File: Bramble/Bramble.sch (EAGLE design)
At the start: 15 parts, among them J3 5787745-1, J4 5787745-1

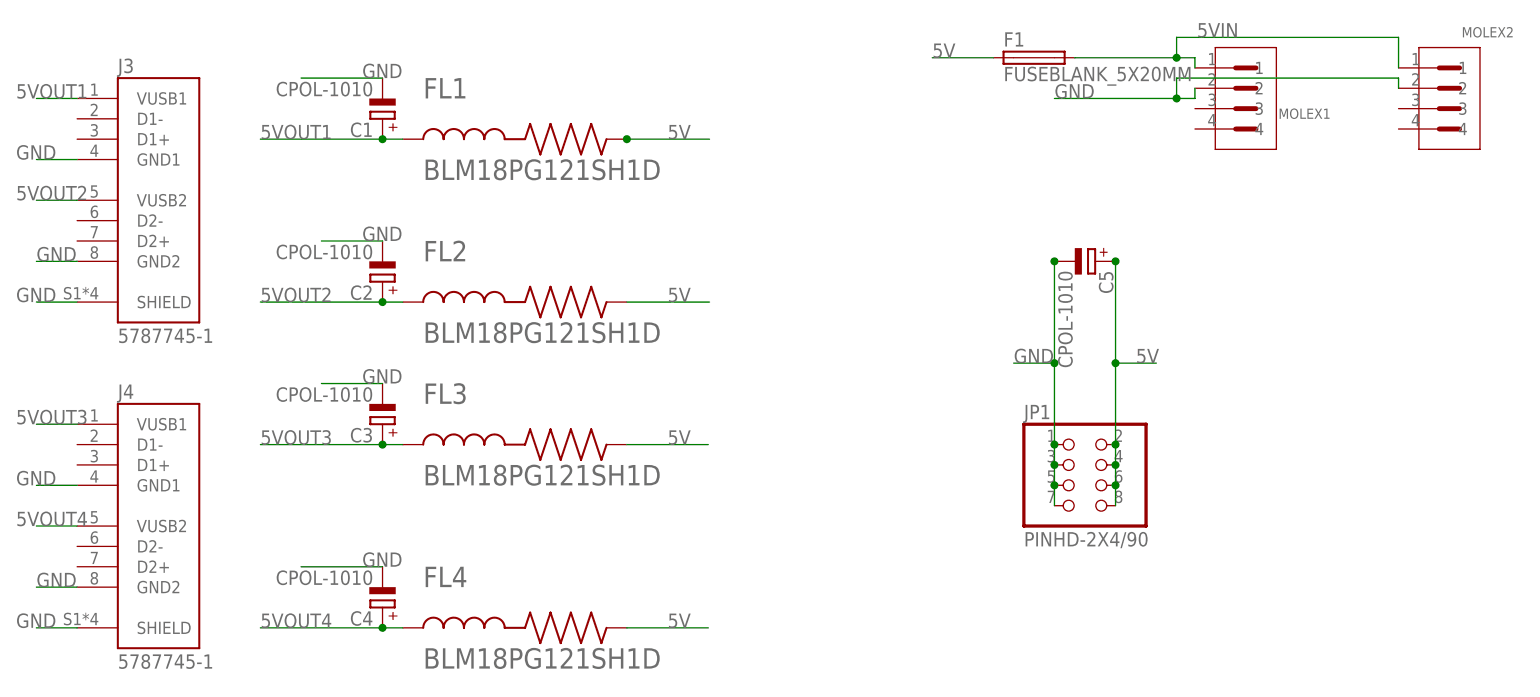
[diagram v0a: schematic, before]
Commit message: joined 1 and 2  aaand 3 and 4
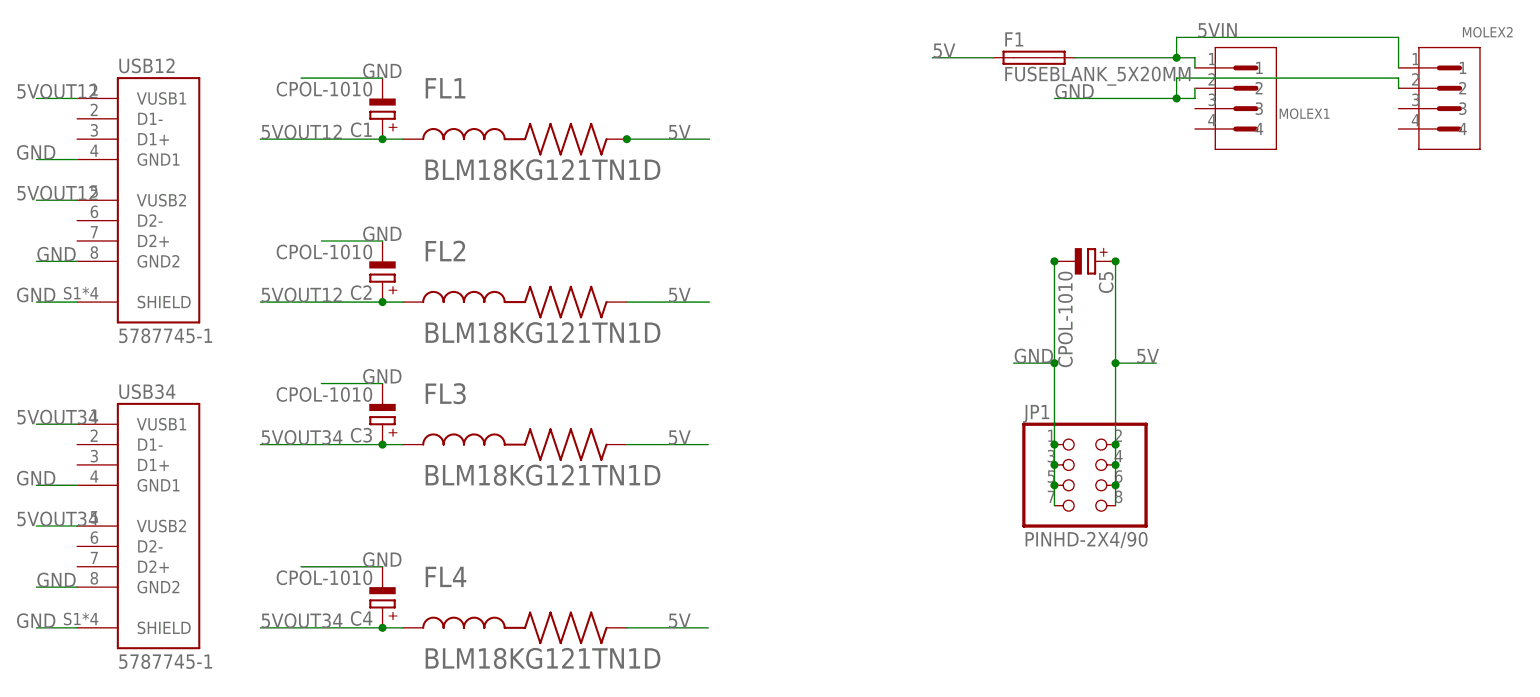
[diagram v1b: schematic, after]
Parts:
- FL1, FL2, FL3, FL4: value BLM18PG121SH1D -> BLM18KG121TN1D
- renumbered J3 to USB12, J4 to USB34
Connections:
- removed net 5VOUT1: C1.+, FL1.1, USB12.VUSB1
- removed net 5VOUT2: C2.+, FL2.1, USB12.VUSB2
- removed net 5VOUT3: C3.+, FL3.1, USB34.VUSB1
- removed net 5VOUT4: C4.+, FL4.1, USB34.VUSB2
- new net 5VOUT12: C1.+, C2.+, FL1.1, FL2.1, USB12.VUSB1, USB12.VUSB2
- new net 5VOUT34: C3.+, C4.+, FL3.1, FL4.1, USB34.VUSB1, USB34.VUSB2
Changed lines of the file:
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@@
 <part name="C4" library="cap-vishay-153clv" deviceset="CPOL-1010" device=""/>
 <part name="C5" library="cap-vishay-153clv" deviceset="CPOL-1010" device=""/>
-<part name="FL1" library="BLM18PG121SH1D" deviceset="BLM18PG121SH1D" device=""/>
-<part name="FL2" library="BLM18PG121SH1D" deviceset="BLM18PG121SH1D" device=""/>
-<part name="FL3" library="BLM18PG121SH1D" deviceset="BLM18PG121SH1D" device=""/>
-<part name="FL4" library="BLM18PG121SH1D" deviceset="BLM18PG121SH1D" device=""/>
+<part name="FL1" library="BLM18PG121SH1D" deviceset="BLM18PG121SH1D" device="" value="BLM18KG121TN1D"/>
+<part name="FL2" library="BLM18PG121SH1D" deviceset="BLM18PG121SH1D" device="" value="BLM18KG121TN1D"/>
+<part name="FL3" library="BLM18PG121SH1D" deviceset="BLM18PG121SH1D" device="" value="BLM18KG121TN1D"/>
+<part name="FL4" library="BLM18PG121SH1D" deviceset="BLM18PG121SH1D" device="" value="BLM18KG121TN1D"/>
 <part name="MOLEX1" library="15244441" deviceset="15244441" device=""/>
 <part name="MOLEX2" library="15244441" deviceset="15244441" device=""/>
-<part name="J3" library="5787745-1" deviceset="5787745-1" device=""/>
-<part name="J4" library="5787745-1" deviceset="5787745-1" device=""/>
+<part name="USB12" library="5787745-1" deviceset="5787745-1" device=""/>
+<part name="USB34" library="5787745-1" deviceset="5787745-1" device=""/>
 </parts>
 <sheets>
@@
 <attribute name="NAME" x="142.23916875" y="76.201240625" size="1.270209375" layer="95"/>
 </instance>
-<instance part="J3" gate="G$1" x="-20.32" y="55.88" smashed="yes">
+<instance part="USB12" gate="G$1" x="-20.32" y="55.88" smashed="yes">
 <attribute name="NAME" x="-25.400109375" y="71.7553" size="1.778040625" layer="95"/>
 <attribute name="VALUE" x="-25.40351875" y="38.0877" size="1.77923125" layer="96"/>
 </instance>
-<instance part="J4" gate="G$1" x="-20.32" y="15.24" smashed="yes">
+<instance part="USB34" gate="G$1" x="-20.32" y="15.24" smashed="yes">
 <attribute name="NAME" x="-25.400109375" y="31.1153" size="1.778040625" layer="95"/>
 <attribute name="VALUE" x="-25.40351875" y="-2.5523" size="1.77923125" layer="96"/>
@@
 <segment>
 <wire x1="-35.56" y1="43.18" x2="-30.48" y2="43.18" width="0.1524" layer="91"/>
-<pinref part="J3" gate="G$1" pin="SHIELD"/>
+<pinref part="USB12" gate="G$1" pin="SHIELD"/>
 <label x="-38.1" y="43.18" size="1.778" layer="95"/>
 </segment>
 <segment>
 <wire x1="-35.56" y1="2.54" x2="-30.48" y2="2.54" width="0.1524" layer="91"/>
-<pinref part="J4" gate="G$1" pin="SHIELD"/>
+<pinref part="USB34" gate="G$1" pin="SHIELD"/>
 <label x="-38.1" y="2.54" size="1.778" layer="95"/>
 </segment>
 <segment>
 <wire x1="-35.56" y1="20.32" x2="-30.48" y2="20.32" width="0.1524" layer="91"/>
-<pinref part="J4" gate="G$1" pin="GND1"/>
+<pinref part="USB34" gate="G$1" pin="GND1"/>
 <label x="-38.1" y="20.32" size="1.778" layer="95"/>
 </segment>
 <segment>
 <wire x1="-35.56" y1="48.26" x2="-30.48" y2="48.26" width="0.1524" layer="91"/>
-<pinref part="J3" gate="G$1" pin="GND2"/>
+<pinref part="USB12" gate="G$1" pin="GND2"/>
 <label x="-35.56" y="48.26" size="1.778" layer="95"/>
 </segment>
 <segment>
 <wire x1="-35.56" y1="60.96" x2="-30.48" y2="60.96" width="0.1524" layer="91"/>
-<pinref part="J3" gate="G$1" pin="GND1"/>
+<pinref part="USB12" gate="G$1" pin="GND1"/>
 <label x="-38.1" y="60.96" size="1.778" layer="95"/>
 </segment>
 <segment>
 <wire x1="-35.56" y1="7.62" x2="-30.48" y2="7.62" width="0.1524" layer="91"/>
-<pinref part="J4" gate="G$1" pin="GND2"/>
+<pinref part="USB34" gate="G$1" pin="GND2"/>
 <label x="-35.56" y="7.62" size="1.778" layer="95"/>
 </segment>
@@
 </segment>
 </net>
-<net name="5VOUT1" class="0">
+<net name="5VOUT12" class="0">
 <segment>
 <wire x1="-35.56" y1="68.58" x2="-30.48" y2="68.58" width="0.1524" layer="91"/>
-<pinref part="J3" gate="G$1" pin="VUSB1"/>
+<pinref part="USB12" gate="G$1" pin="VUSB1"/>
 <label x="-38.1" y="68.58" size="1.778" layer="95"/>
+</segment>
+<segment>
+<wire x1="-35.56" y1="55.88" x2="-30.48" y2="55.88" width="0.1524" layer="91"/>
+<pinref part="USB12" gate="G$1" pin="VUSB2"/>
+<label x="-38.1" y="55.88" size="1.778" layer="95"/>
 </segment>
 <segment>
@@
 <label x="-7.62" y="63.5" size="1.778" layer="95"/>
 </segment>
-</net>
-<net name="5VOUT2" class="0">
-<segment>
-<wire x1="-35.56" y1="55.88" x2="-30.48" y2="55.88" width="0.1524" layer="91"/>
-<pinref part="J3" gate="G$1" pin="VUSB2"/>
-<label x="-38.1" y="55.88" size="1.778" layer="95"/>
-</segment>
 <segment>
 <wire x1="-7.62" y1="43.18" x2="7.62" y2="43.18" width="0.1524" layer="91"/>
@@
 </segment>
 </net>
-<net name="5VOUT3" class="0">
+<net name="5VOUT34" class="0">
 <segment>
 <wire x1="-35.56" y1="27.94" x2="-30.48" y2="27.94" width="0.1524" layer="91"/>
-<pinref part="J4" gate="G$1" pin="VUSB1"/>
+<pinref part="USB34" gate="G$1" pin="VUSB1"/>
 <label x="-38.1" y="27.94" size="1.778" layer="95"/>
 </segment>
@@
 <label x="-7.62" y="25.4" size="1.778" layer="95"/>
 </segment>
-</net>
-<net name="5VOUT4" class="0">
 <segment>
 <wire x1="-35.56" y1="15.24" x2="-30.48" y2="15.24" width="0.1524" layer="91"/>
-<pinref part="J4" gate="G$1" pin="VUSB2"/>
+<pinref part="USB34" gate="G$1" pin="VUSB2"/>
 <label x="-38.1" y="15.24" size="1.778" layer="95"/>
 </segment>
